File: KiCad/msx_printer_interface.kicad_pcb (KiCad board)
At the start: 2 copper layers, 65.7 x 54 mm, 12 parts, among them J1 MSX Cartridge Connector, J2 Conn_02x07_Top_Bottom, U1 ATF22V10C-15PU, U2 74HC273

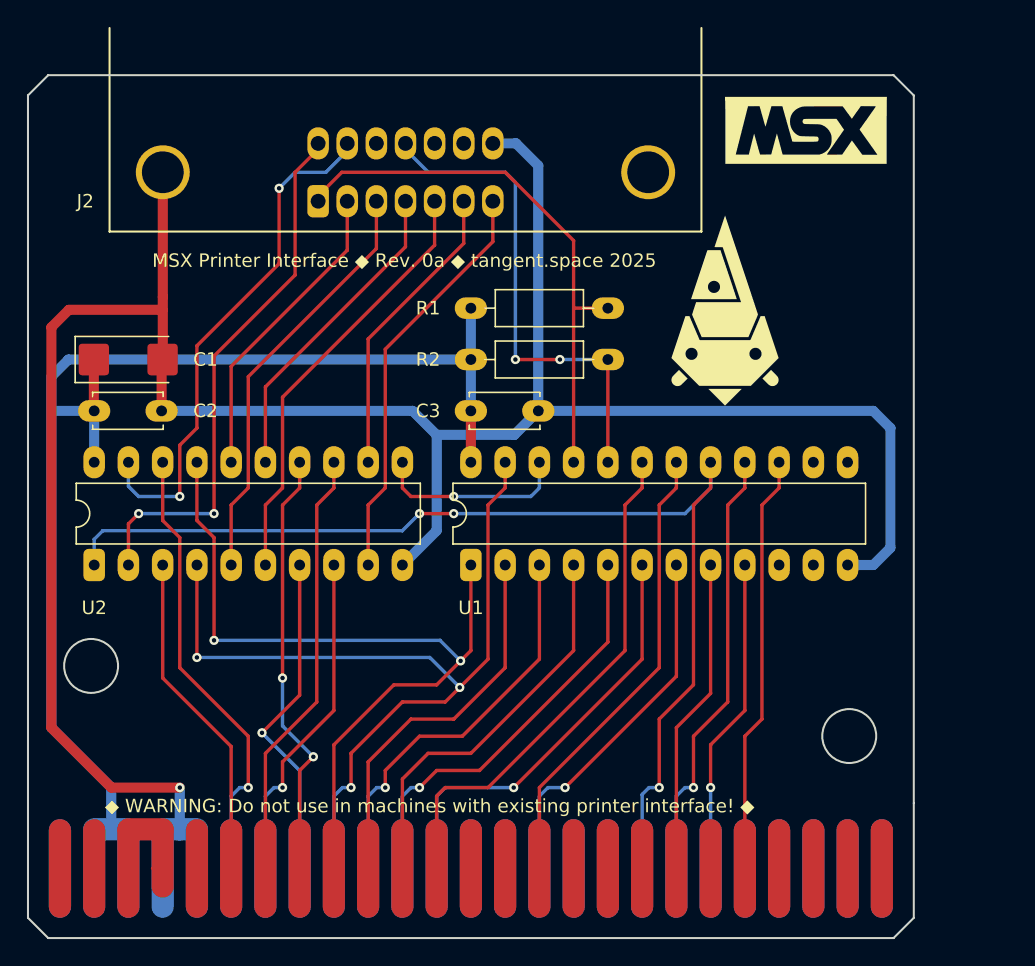
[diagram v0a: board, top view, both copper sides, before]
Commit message: Update msx_printer_interface.kicad_pcb
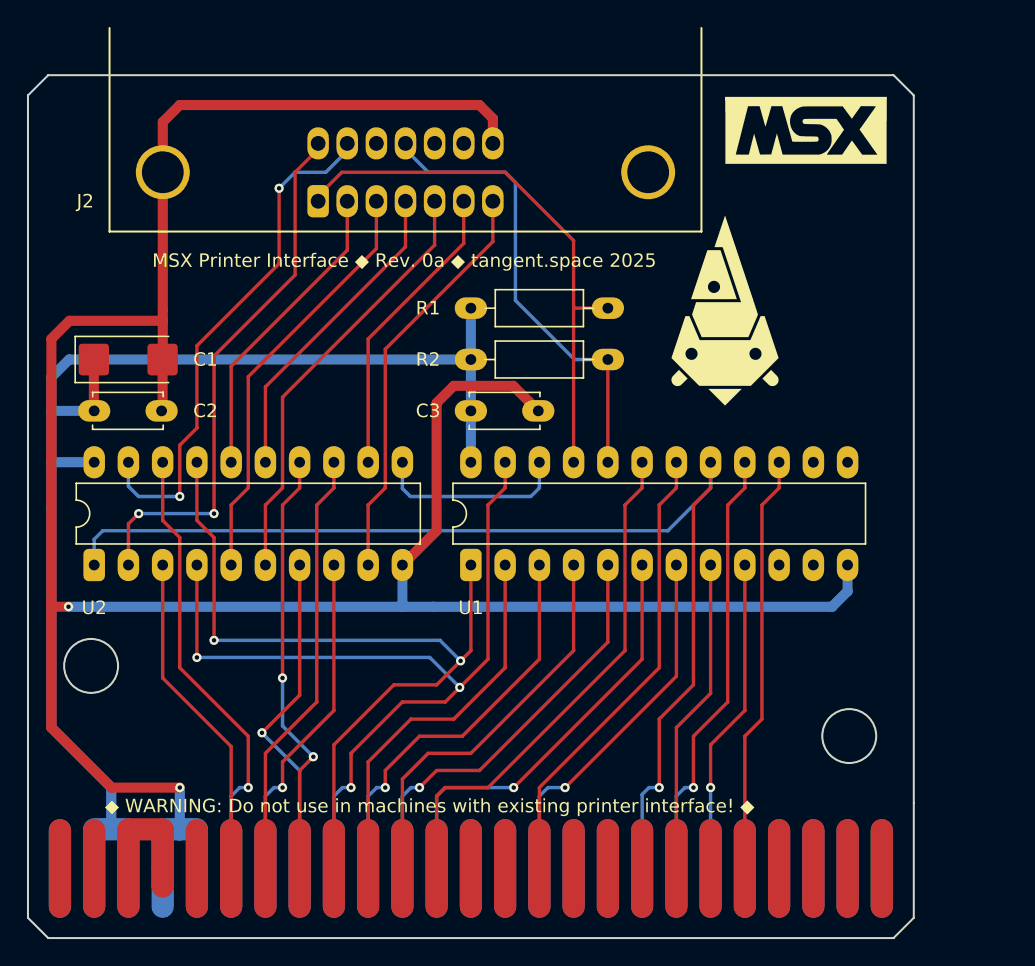
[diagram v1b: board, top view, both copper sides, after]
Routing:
- net GND: track 174.7 -> 189.7 mm, vias 1 -> 2
- net BUSY: track 36.8 -> 34.2 mm, vias 2 -> 0
- net CLK_DATA: vias 1 -> 0
- net #RESET: vias 3 -> 1
